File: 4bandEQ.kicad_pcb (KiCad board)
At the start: 2 copper layers, 35.6 x 147.3 mm, 70 parts, among them J1 EQ_IN, J2 EQ_OUT, J3 PWR_IN, SW1 MF1_IN, SW2 MF2_IN, SW3 ML5000, SW4 ML5000, SW5 ML5000, SW6 ML5000, U1 TL072, U2 TL072, U3 TL072

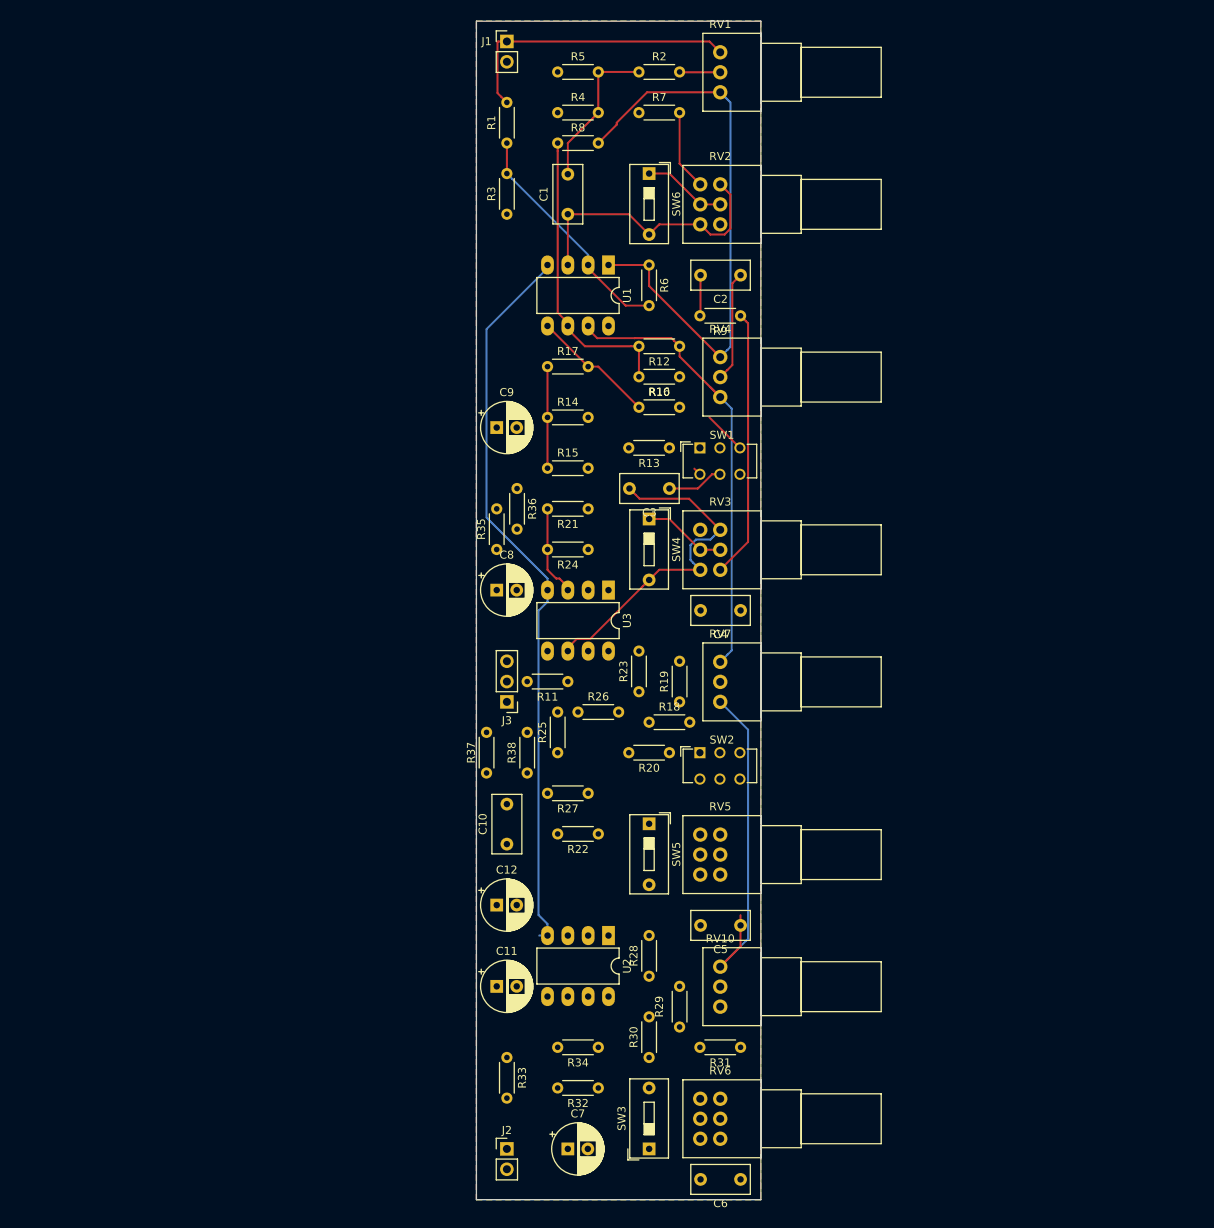
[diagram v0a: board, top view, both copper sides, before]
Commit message: layout board
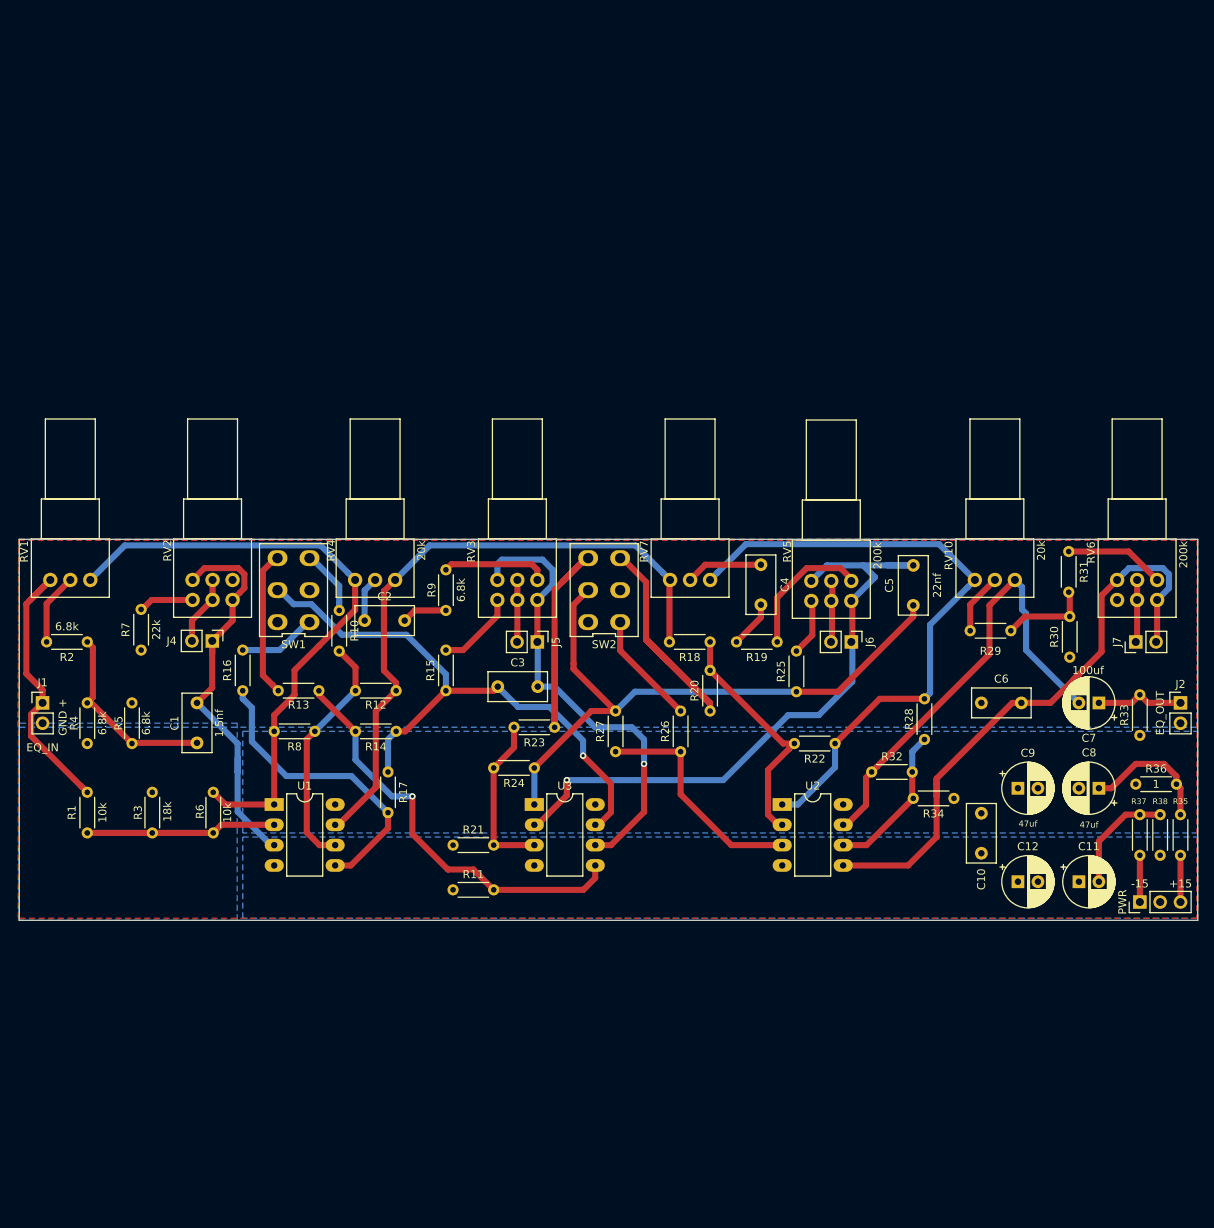
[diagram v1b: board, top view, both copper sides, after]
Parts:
- removed SW3, SW4, SW5, SW6: ML5000, Button_Switch_THT:SW_DIP_SPSTx01_Slide_9.78x4.72mm_W7.62mm_P2.54mm
- added J4: H_JMP, Connector_PinHeader_2.54mm:PinHeader_1x02_P2.54mm_Vertical, F.Cu at (94.0, 97.8)
- added J5: MF1_JMP, Connector_PinHeader_2.54mm:PinHeader_1x02_P2.54mm_Vertical, F.Cu at (134.6, 97.9)
- added J6: MF2_JMP, Connector_PinHeader_2.54mm:PinHeader_1x02_P2.54mm_Vertical, F.Cu at (173.9, 97.9)
- added J7: LF_JMP, Connector_PinHeader_2.54mm:PinHeader_1x02_P2.54mm_Vertical, F.Cu at (209.4, 97.9)
- J3: value PWR_IN -> PWR
- SW1, SW2: footprint Button_Switch_THT:SW_CuK_JS202011CQN_DPDT_Straight -> F2UEE-TB_PUSHBTN:PB_SW_F2UEE
- moved J1 101.0 mm to (72.8, 105.5)
- moved J2 101.0 mm to (215.0, 105.5)
- moved R1 100.9 mm to (78.4, 121.8)
- moved RV1 99.6 mm to (78.7, 90.2), turned to 90 degrees
- moved R2 99.2 mm to (78.4, 97.9), turned to 180 degrees
- moved R4 98.4 mm to (78.4, 110.6), turned to 90 degrees
- moved R5 95.1 mm to (83.9, 105.5), turned to 270 degrees
- moved R35 91.7 mm to (215.0, 119.5), turned to 270 degrees
- moved R7 91.6 mm to (85.1, 98.9), turned to 90 degrees
- moved R33 88.8 mm to (209.9, 109.6), turned to 90 degrees
- moved RV6 88.7 mm to (212.1, 90.2), turned to 90 degrees
- moved C7 86.7 mm to (204.8, 105.5), turned to 180 degrees
- moved R36 85.7 mm to (209.4, 115.7), turned to 0 degrees
- moved R6 85.5 mm to (94.1, 116.7)
- moved R3 84.8 mm to (86.5, 116.7), turned to 270 degrees
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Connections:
- J3 pad 2: +15V -> GND
- J3 pad 3: GND -> +15V
- RV2 pad 1: (no net) -> Net-(RV2-Pad1)
- RV6 pad 6: (no net) -> Net-(RV6-Pad6)
- SW1 pad 6: (no net) -> Net-(SW1-Pad6)
- SW2 pad 6: (no net) -> Net-(SW2-Pad6)
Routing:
- net -VC: track 92.1 -> 0.00 mm
- net Net-(C5-Pad2): track 0.00 -> 81.3 mm, vias 0 -> 1
- net Net-(C5-Pad1): track 0.00 -> 79.2 mm
- net Net-(C6-Pad2): track 0.00 -> 76.3 mm
- net Net-(C7-Pad2): track 0.00 -> 58.4 mm
- net Net-(C3-Pad1): track 19.7 -> 74.5 mm, vias 0 -> 1
- net Net-(R11-Pad2): track 0.00 -> 52.2 mm, vias 0 -> 1
- net Net-(R22-Pad1): track 43.5 -> 84.2 mm
- net Net-(R20-Pad1): track 0.00 -> 39.1 mm
- net Net-(R23-Pad1): track 0.00 -> 37.3 mm
- net Net-(R18-Pad1): track 0.00 -> 30.4 mm
- net Net-(R26-Pad1): track 0.00 -> 28.8 mm
- net Net-(R12-Pad1): track 57.3 -> 81.2 mm
- net Net-(R16-Pad1): track 15.6 -> 38.0 mm
- net Net-(R9-Pad1): track 33.6 -> 13.3 mm
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- added copper zone on B.Cu, net -VC
- added copper zone on B.Cu, net GND
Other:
- board size 35.6 x 147.3 mm -> 147.3 x 47.6 mm
- board text added: "+"
- board text added: "+15"
- board text added: "-15"
- board text added: "GND"

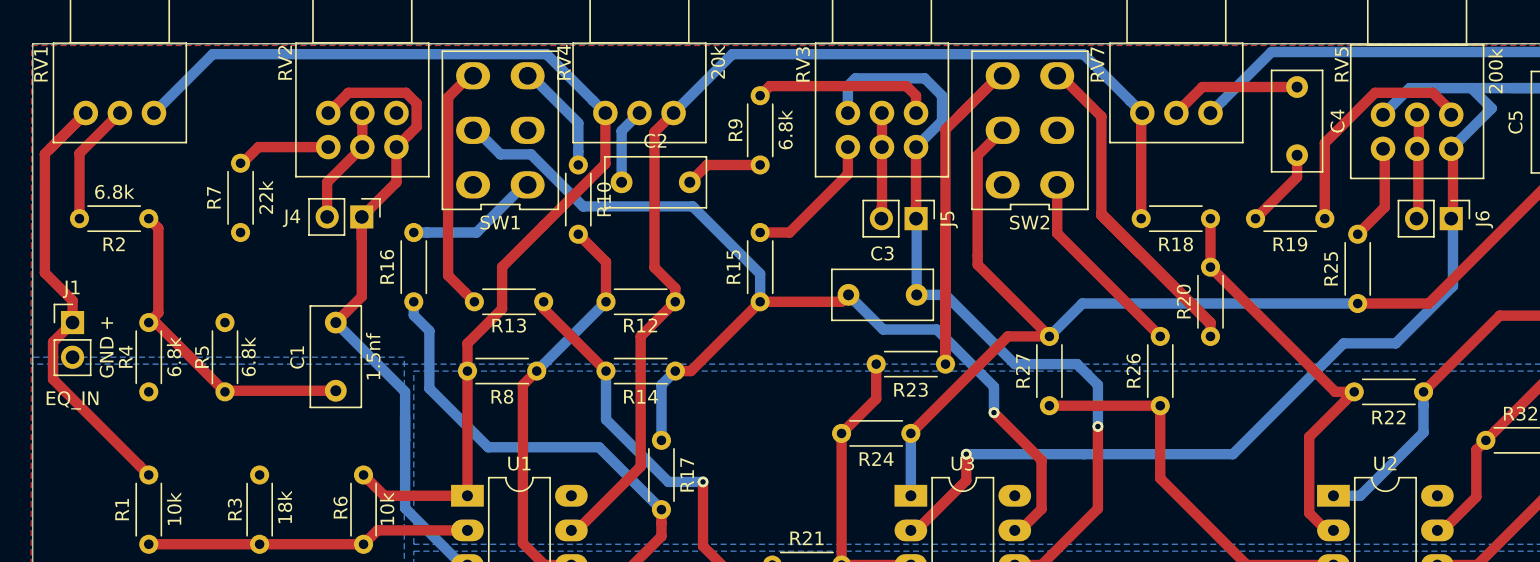
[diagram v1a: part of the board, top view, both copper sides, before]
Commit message: update
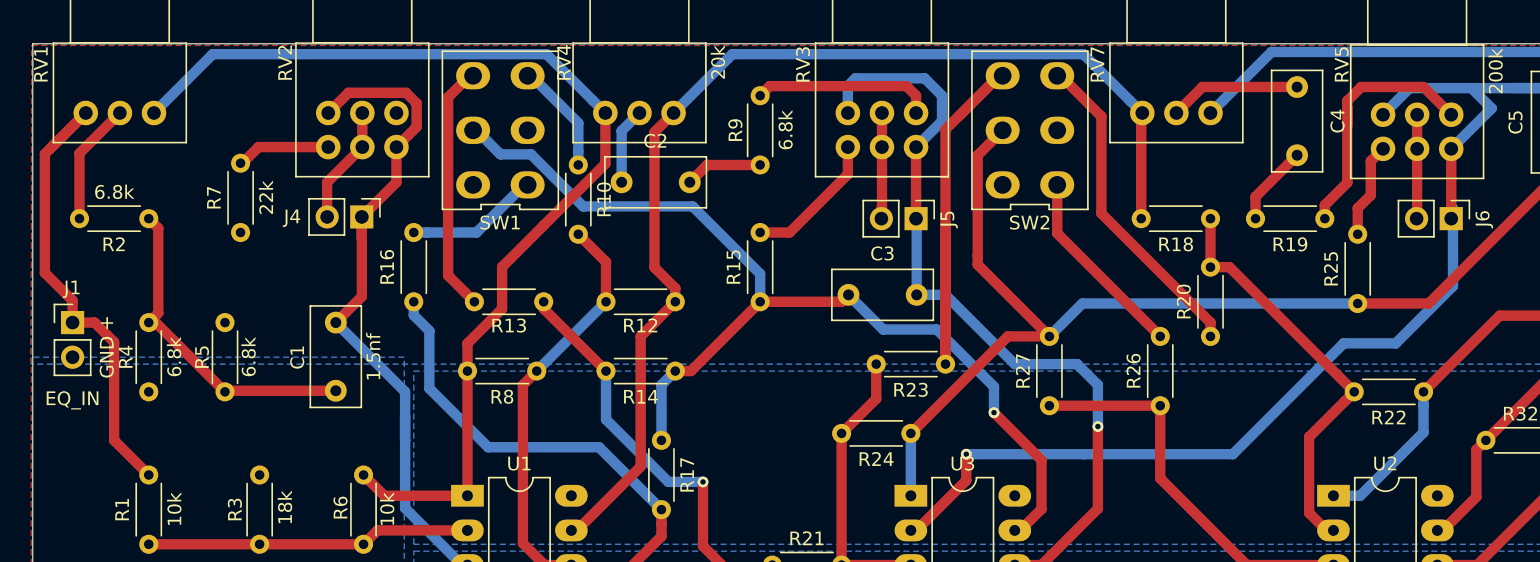
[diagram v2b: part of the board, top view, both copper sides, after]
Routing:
- net Net-(R20-Pad1): track 39.1 -> 23.9 mm
- net Net-(R19-Pad1): track 17.1 -> 20.0 mm
- net Net-(J6-Pad2): track 7.00 -> 7.69 mm
- net Net-(C5-Pad2): track 81.3 -> 81.9 mm
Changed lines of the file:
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@@
-(kicad_pcb (version 20171130) (host pcbnew "(5.1.4-0-10_14)")
+(kicad_pcb (version 20171130) (host pcbnew "(5.1.5-0-10_14)")
   (general
     (thickness 1.6)
     (drawings 8)
-    (tracks 331)
+    (tracks 336)
     (zones 0)
     (modules 70)
@@
   (segment (start 123.19 104.013) (end 123.19 101.96702) (width 0.762) (layer B.Cu) (net 6))
   (segment (start 118.24399 97.02101) (end 110.206895 97.02101) (width 0.762) (layer B.Cu) (net 6))
-  (segment (start 162.56 94.869) (end 159.512 97.917) (width 0.762) (layer F.Cu) (net 7))
-  (segment (start 162.56 93.265) (end 162.56 94.869) (width 0.762) (layer F.Cu) (net 7))
+  (segment (start 159.512 96.313) (end 159.512 97.917) (width 0.762) (layer F.Cu) (net 7))
+  (segment (start 162.56 93.265) (end 159.512 96.313) (width 0.762) (layer F.Cu) (net 7))
   (segment (start 155.615 88.265) (end 162.56 88.265) (width 0.762) (layer F.Cu) (net 8))
   (segment (start 153.71 90.17) (end 155.615 88.265) (width 0.762) (layer F.Cu) (net 8))
-  (segment (start 173.99 97.155) (end 173.99 92.67) (width 0.762) (layer F.Cu) (net 9))
   (segment (start 181.61 88.345) (end 178.315 88.345) (width 0.762) (layer B.Cu) (net 9))
   (segment (start 170.815 88.345) (end 168.99 90.17) (width 0.762) (layer B.Cu) (net 9))
@@
   (segment (start 173.99 102.87) (end 169.799 107.061) (width 0.762) (layer B.Cu) (net 9))
   (segment (start 173.99 97.155) (end 173.99 102.87) (width 0.762) (layer B.Cu) (net 9))
+  (segment (start 173.863 92.797) (end 173.863 97.917) (width 0.762) (layer F.Cu) (net 9))
   (segment (start 139.13899 93.27101) (end 140.97 91.44) (width 0.762) (layer F.Cu) (net 10))
   (segment (start 134.239 118.237) (end 134.239 113.665) (width 0.762) (layer B.Cu) (net 10))
@@
   (segment (start 70.739 93.171) (end 70.739 101.893) (width 0.762) (layer F.Cu) (net 15))
   (segment (start 73.74 90.17) (end 70.739 93.171) (width 0.762) (layer F.Cu) (net 15))
-  (segment (start 71.339999 109.693999) (end 77.659001 116.013001) (width 0.762) (layer F.Cu) (net 15))
-  (segment (start 77.659001 116.013001) (end 78.359 116.713) (width 0.762) (layer F.Cu) (net 15))
-  (segment (start 71.339999 106.968001) (end 71.339999 109.693999) (width 0.762) (layer F.Cu) (net 15))
-  (segment (start 72.771 105.537) (end 71.339999 106.968001) (width 0.762) (layer F.Cu) (net 15))
+  (segment (start 74.383 105.537) (end 75.819 106.973) (width 0.762) (layer F.Cu) (net 15))
+  (segment (start 72.771 105.537) (end 74.383 105.537) (width 0.762) (layer F.Cu) (net 15))
+  (segment (start 75.819 114.173) (end 78.359 116.713) (width 0.762) (layer F.Cu) (net 15))
+  (segment (start 75.819 106.973) (end 75.819 114.173) (width 0.762) (layer F.Cu) (net 15))
   (segment (start 95.123 120.777) (end 94.107 121.793) (width 0.762) (layer F.Cu) (net 16))
   (segment (start 101.727 120.777) (end 95.123 120.777) (width 0.762) (layer F.Cu) (net 16))
@@
   (segment (start 164.721198 120.777) (end 163.445999 119.501801) (width 0.762) (layer F.Cu) (net 29))
   (segment (start 165.227 120.777) (end 164.721198 120.777) (width 0.762) (layer F.Cu) (net 29))
-  (segment (start 165.354 110.617) (end 156.21 101.473) (width 0.762) (layer F.Cu) (net 29))
-  (segment (start 166.751 110.617) (end 165.354 110.617) (width 0.762) (layer F.Cu) (net 29))
   (segment (start 156.21 101.473) (end 156.21 97.917) (width 0.762) (layer F.Cu) (net 29))
-  (segment (start 172.508999 88.688999) (end 173.99 90.17) (width 0.762) (layer F.Cu) (net 30))
-  (segment (start 168.279119 88.688999) (end 172.508999 88.688999) (width 0.762) (layer F.Cu) (net 30))
-  (segment (start 164.592 92.376118) (end 168.279119 88.688999) (width 0.762) (layer F.Cu) (net 30))
-  (segment (start 164.592 97.917) (end 164.592 92.376118) (width 0.762) (layer F.Cu) (net 30))
-  (segment (start 151.003 100.457) (end 148.209 97.663) (width 0.762) (layer F.Cu) (net 31))
+  (segment (start 157.607 101.473) (end 156.21 101.473) (width 0.762) (layer F.Cu) (net 29))
+  (segment (start 166.751 110.617) (end 157.607 101.473) (width 0.762) (layer F.Cu) (net 29))
+  (segment (start 167.259 88.265) (end 166.243 89.281) (width 0.762) (layer F.Cu) (net 30))
+  (segment (start 173.863 90.297) (end 171.831 88.265) (width 0.762) (layer F.Cu) (net 30))
+  (segment (start 171.831 88.265) (end 167.259 88.265) (width 0.762) (layer F.Cu) (net 30))
+  (segment (start 166.243 91.059) (end 166.243 90.551) (width 0.762) (layer F.Cu) (net 30))
+  (segment (start 166.243 95.276051) (end 166.243 89.789) (width 0.762) (layer F.Cu) (net 30))
+  (segment (start 164.592 96.927051) (end 166.243 95.276051) (width 0.762) (layer F.Cu) (net 30))
+  (segment (start 164.592 97.917) (end 164.592 96.927051) (width 0.762) (layer F.Cu) (net 30))
+  (segment (start 166.243 89.789) (end 166.243 91.059) (width 0.762) (layer F.Cu) (net 30))
+  (segment (start 166.243 89.281) (end 166.243 89.789) (width 0.762) (layer F.Cu) (net 30))
   (segment (start 145.22 87.44) (end 144.97 87.44) (width 0.762) (layer F.Cu) (net 31))
   (segment (start 148.209 90.429) (end 145.22 87.44) (width 0.762) (layer F.Cu) (net 31))
-  (segment (start 156.083 105.537) (end 148.209 97.663) (width 0.762) (layer F.Cu) (net 31))
   (segment (start 156.21 105.537) (end 148.209 97.536) (width 0.762) (layer F.Cu) (net 31))
   (segment (start 148.209 97.536) (end 148.209 90.429) (width 0.762) (layer F.Cu) (net 31))
   (segment (start 156.21 106.553) (end 156.21 105.537) (width 0.762) (layer F.Cu) (net 31))
-  (segment (start 148.209 97.663) (end 148.209 97.536) (width 0.762) (layer F.Cu) (net 31))
   (segment (start 134.239 123.317) (end 129.159 123.317) (width 0.762) (layer F.Cu) (net 32))
   (segment (start 129.159 123.317) (end 129.159 113.665) (width 0.762) (layer F.Cu) (net 32))
@@
   (segment (start 140.72 87.44) (end 136.779 91.381) (width 0.762) (layer F.Cu) (net 34))
   (segment (start 140.97 87.44) (end 140.72 87.44) (width 0.762) (layer F.Cu) (net 34))
-  (segment (start 168.99 97.075) (end 167.005 99.06) (width 0.762) (layer F.Cu) (net 35))
-  (segment (start 168.99 92.67) (end 168.99 97.075) (width 0.762) (layer F.Cu) (net 35))
+  (segment (start 167.963001 93.696999) (end 167.963001 96.196999) (width 0.762) (layer F.Cu) (net 35))
+  (segment (start 168.863 92.797) (end 167.963001 93.696999) (width 0.762) (layer F.Cu) (net 35))
+  (segment (start 167.005 97.155) (end 167.005 99.06) (width 0.762) (layer F.Cu) (net 35))
+  (segment (start 167.963001 96.196999) (end 167.005 97.155) (width 0.762) (layer F.Cu) (net 35))
   (segment (start 145.415 95.885) (end 144.97 95.44) (width 0.762) (layer F.Cu) (net 36))
   (segment (start 144.97 98.996) (end 144.97 95.44) (width 0.762) (layer F.Cu) (net 36))
@@
   (segment (start 132.12 92.67) (end 132.12 97.115) (width 0.762) (layer F.Cu) (net 53))
   (segment (start 171.45 92.71) (end 171.49 92.67) (width 0.762) (layer F.Cu) (net 54))
-  (segment (start 171.45 97.155) (end 171.45 92.71) (width 0.762) (layer F.Cu) (net 54))
-  (segment (start 171.49 92.67) (end 171.49 90.17) (width 0.762) (layer F.Cu) (net 54))
+  (segment (start 171.363 97.877) (end 171.323 97.917) (width 0.762) (layer F.Cu) (net 54))
+  (segment (start 171.363 92.797) (end 171.363 97.877) (width 0.762) (layer F.Cu) (net 54))
+  (segment (start 171.363 92.797) (end 171.363 90.297) (width 0.762) (layer F.Cu) (net 54))
   (segment (start 209.59 97.115) (end 209.55 97.155) (width 0.762) (layer F.Cu) (net 55))
   (segment (start 209.59 92.67) (end 209.59 97.115) (width 0.762) (layer F.Cu) (net 55))
